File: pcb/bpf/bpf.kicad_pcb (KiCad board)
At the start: 2 copper layers, 58 x 53 mm, 21 parts, among them J1 input, J2 power_input, J3 audio_out, U1 TI080, U2 TI080

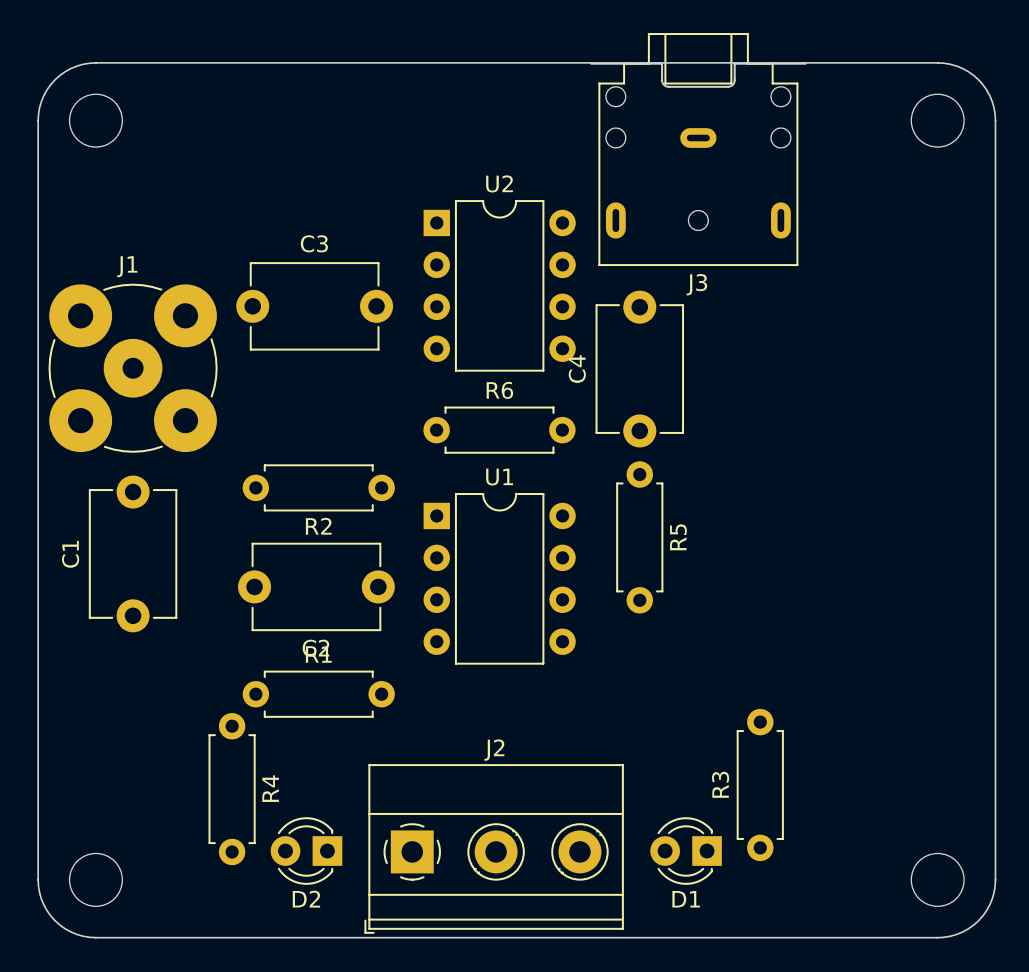
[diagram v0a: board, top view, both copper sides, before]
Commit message: finalize layout and routing
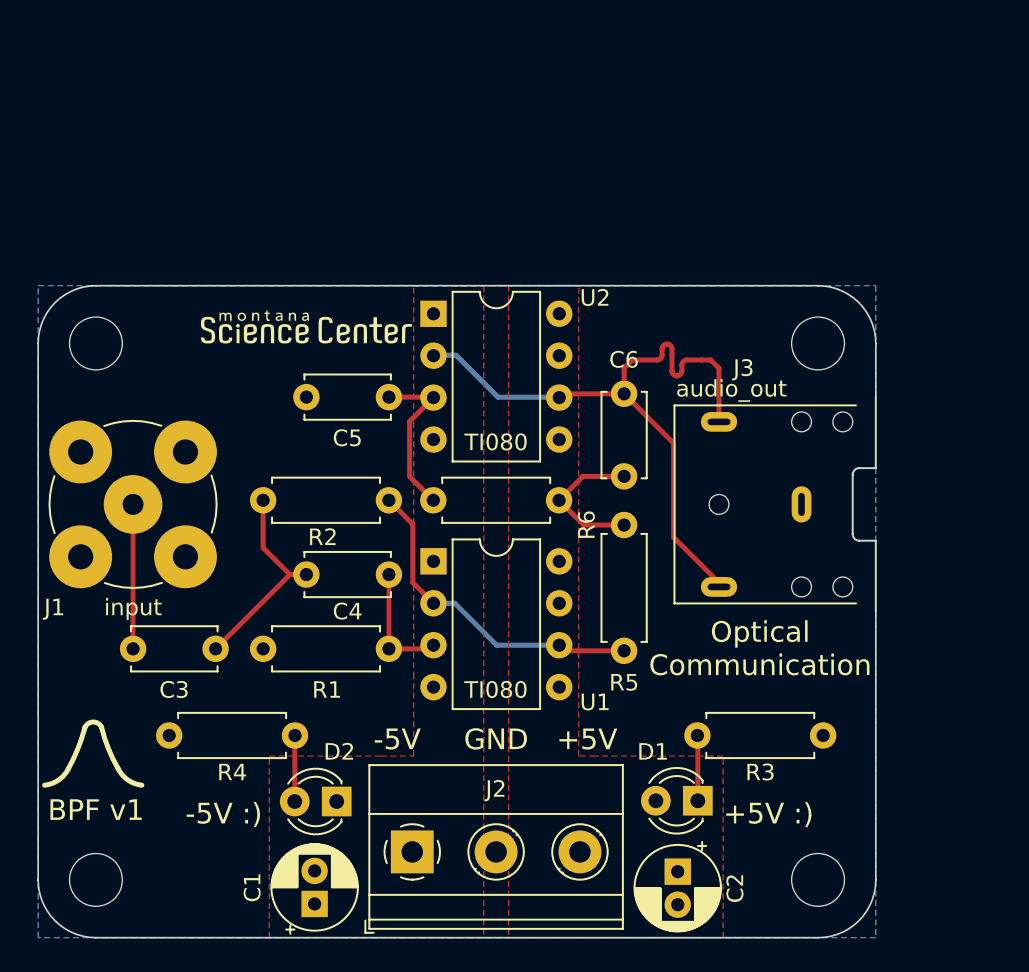
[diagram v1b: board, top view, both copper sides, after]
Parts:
- added C1: 1uF, Capacitor_THT:CP_Radial_D5.0mm_P2.00mm, F.Cu at (91.8, 128.0)
- added C2: 1uF, Capacitor_THT:CP_Radial_D5.0mm_P2.00mm, F.Cu at (113.8, 126.0)
- added G***: LOGO, msc-logos:msc-gears-soldermask-5mm, F.Cu at (83.2, 92.8)
- added G***: LOGO, msc-logos:msc-text-silkscreen, F.Cu at (91.2, 93.0)
- C3: renamed from C1; footprint Capacitor_THT:C_Disc_D7.5mm_W5.0mm_P7.50mm -> Capacitor_THT:C_Disc_D5.0mm_W2.5mm_P5.00mm
- C4: renamed from C2; footprint Capacitor_THT:C_Disc_D7.5mm_W5.0mm_P7.50mm -> Capacitor_THT:C_Disc_D5.0mm_W2.5mm_P5.00mm
- C5: renamed from C3; footprint Capacitor_THT:C_Disc_D7.5mm_W5.0mm_P7.50mm -> Capacitor_THT:C_Disc_D5.0mm_W2.5mm_P5.00mm
- C6: renamed from C4; footprint Capacitor_THT:C_Disc_D7.5mm_W5.0mm_P7.50mm -> Capacitor_THT:C_Disc_D5.0mm_W2.5mm_P5.00mm
- R1: value 22k ohms -> 22k
- R2, R5, R6: value 11k ohms -> 11k
- moved J3 23.1 mm to (121.2, 103.8), turned to 90 degrees
- moved H3 15.3 mm to (122.2, 94.0)
- moved H2 13.5 mm to (78.5, 94.0)
- moved J1 8.25 mm to (80.8, 103.8)
- moved R3 7.80 mm to (114.9, 117.8), turned to 0 degrees
- moved H1 7.25 mm to (122.2, 126.5)
- moved C5 6.39 mm to (91.2, 97.2)
- moved U2 5.50 mm to (99.0, 92.2)
- moved C3 5.39 mm to (85.8, 112.5), turned to 180 degrees
- moved R6 4.25 mm to (98.9, 103.5)
- moved R4 3.85 mm to (90.6, 117.8), turned to 180 degrees
- moved R5 3.20 mm to (110.5, 105.0)
- moved D1 3.10 mm to (115.0, 121.7)
- moved D2 3.05 mm to (93.1, 121.8)
- moved C6 2.91 mm to (110.5, 102.0)
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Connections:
- R4 pad 1: GND -> Net-(D2-Pad2)
- R4 pad 2: Net-(D2-Pad2) -> GND
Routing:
- net Net-(C6-Pad2): track 0.00 -> 40.8 mm
- net Net-(R2-Pad1): track 0.00 -> 20.1 mm
- net Net-(C3-Pad1): track 0.00 -> 12.5 mm
- net Net-(C5-Pad2): track 0.00 -> 10.1 mm
- net Net-(C6-Pad1): track 0.00 -> 9.10 mm
- net Net-(C3-Pad2): track 0.00 -> 9.00 mm
- net Net-(C4-Pad1): track 0.00 -> 7.29 mm
- net Net-(D2-Pad2): track 0.00 -> 4.01 mm
- net Net-(D1-Pad1): track 0.00 -> 3.97 mm
- added copper zone on F.Cu, net +5V
- added copper zone on F.Cu, net -5V
- added copper zone on B.Cu, net GND
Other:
- board size 58 x 53 mm -> 50.8 x 39.5 mm
- board text added: "+5V"
- board text added: "+5V :)"
- board text added: "-5V"
- board text added: "-5V :)"
- board text added: "BPF v1"
- board text added: "GND"
- board text added: "Optical Communication"
